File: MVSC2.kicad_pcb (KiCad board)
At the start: 4 copper layers, 68.3 x 95.1 mm, 291 parts, among them J1 USB_C-SIGNAL, J10 PWM3_OUT, J11 PWM_IN, J12 HSES, J16 ADC0, J17 ESTP0, J18 ESTP1, J19 ESTP2, J2 EXP0, J20 ESTP3, J21 ESTP4, J22 ESTP5, J23 POWER, J25 SERV0, J26 SERV1, J29 ADC1, J3 EXP1, J30 HSES, J31 HSES, J32 HSES, J4 EXPB, J5 HSES, J6 PWM0_OUT, J7 PWM1_OUT, J8 HSES, J9 PWM2_OUT, P1 STP0, P2 STP2, P3 STP4, P4 STP1, P5 STP3, P6 STP5, P9 UART, Q1 AO3400A, Q10 AO3400A, Q2 AO3400A, Q3 AO3400A, Q4 AO3400A, Q5 AO3400A, Q6 AO3400A, SW1 SKRKAEE020, SW2 SKRKAEE020, U1 XC6206P332MR, U10 TMC2208-LA-T, U11 TMC2208-LA-T, U12 TMC2208-LA-T, U13 CH912LSR, U14 CH912LSR, U2 CH912LSR, U3 STM32F411RET6, U4 CH912LSR, U5 TMC2208-LA-T, U6 TMC2208-LA-T, U7 TMC2208-LA-T, U8 CH912LSR, U9 CH912LSR, Y1 25MHZ 12pF, Y2 32.768KHz 12.5pF

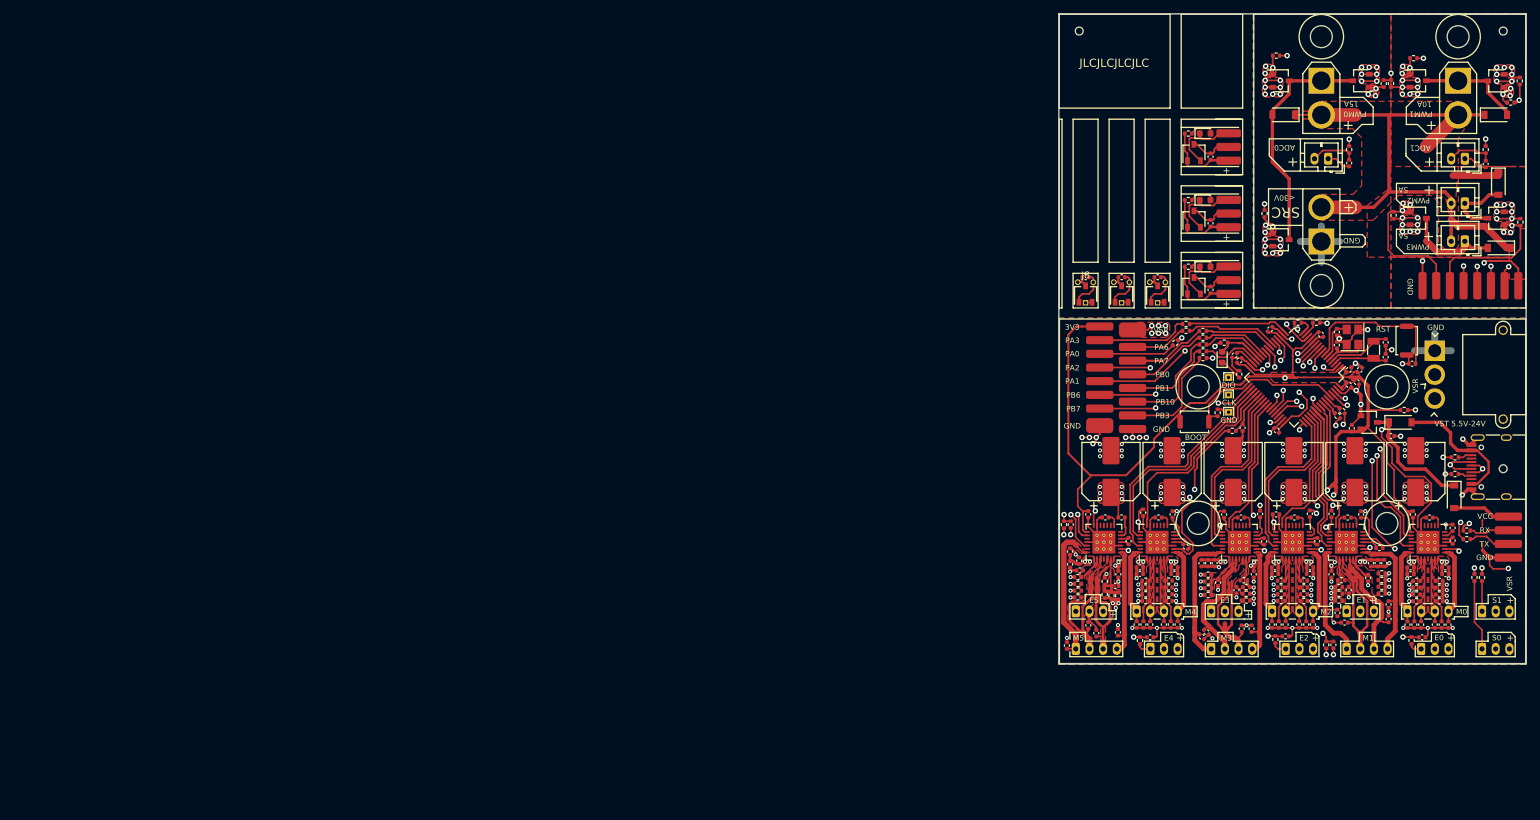
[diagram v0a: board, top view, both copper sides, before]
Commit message: going to rearrange everything
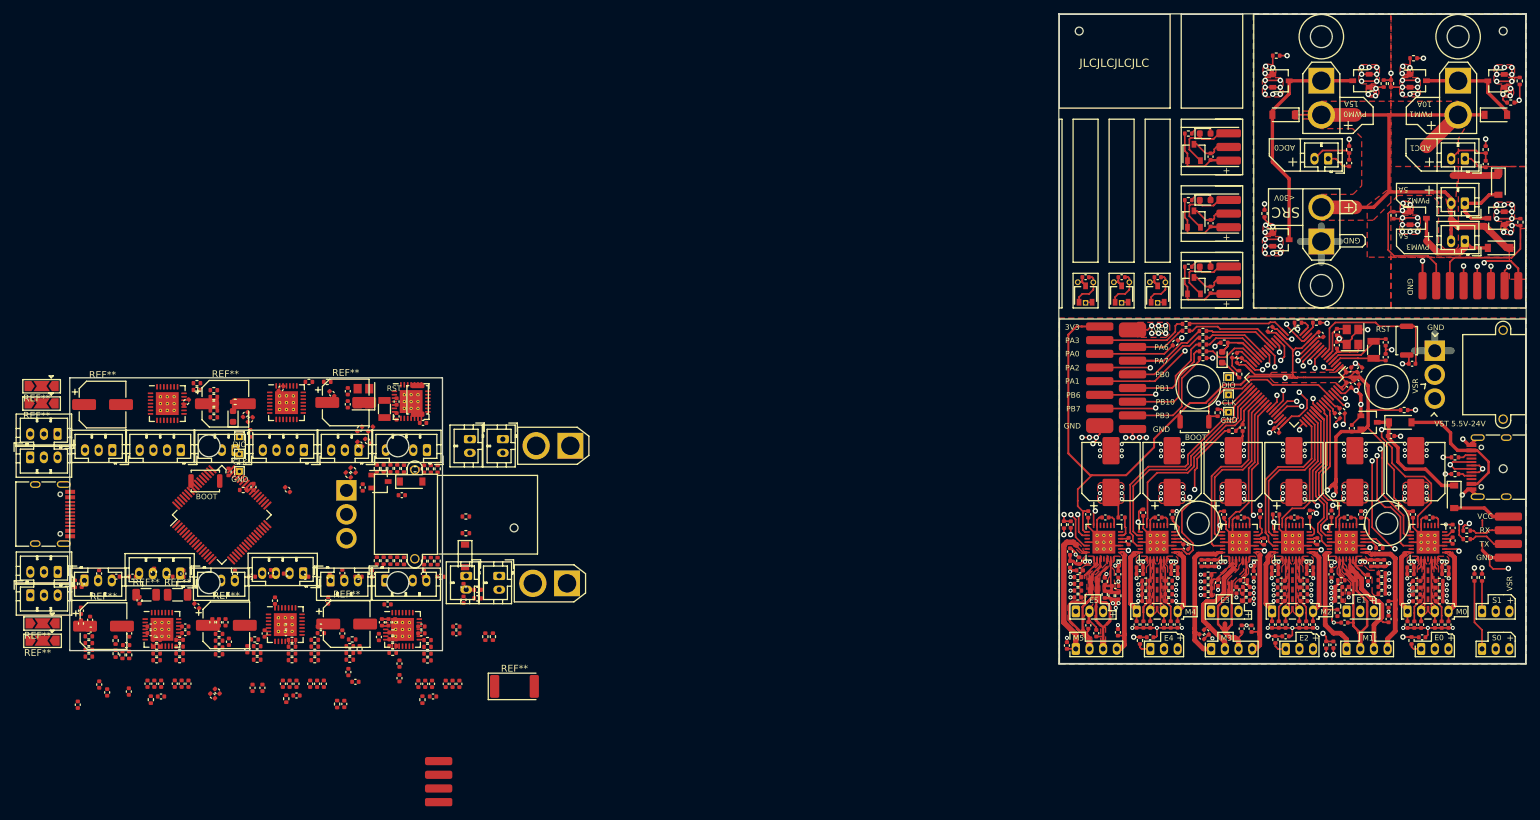
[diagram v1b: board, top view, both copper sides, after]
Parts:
- added C1: 1.0uF 25V, Capacitor_SMD:C_0402_1005Metric, F.Cu at (20.9, 145.9)
- added C10: 4.7uF 10V, Capacitor_SMD:C_0402_1005Metric, F.Cu at (-1.93, 134.1)
- added C100: 470pF 50V, Capacitor_SMD:C_0402_1005Metric, F.Cu at (-26.4, 176.5)
- added C101: 470pF 50V, Capacitor_SMD:C_0402_1005Metric, F.Cu at (-19.0, 174.6)
- added C102: 470pF 50V, Capacitor_SMD:C_0402_1005Metric, F.Cu at (14.2, 173.2)
- added C103: 470pF 50V, Capacitor_SMD:C_0402_1005Metric, F.Cu at (20.6, 172.6)
- added C104: 470pF 50V, Capacitor_SMD:C_0402_1005Metric, F.Cu at (-6.04, 174.5)
- added C105: 470pF 50V, Capacitor_SMD:C_0402_1005Metric, F.Cu at (-0.88, 174.0)
- added C106: 470pF 50V, Capacitor_SMD:C_0402_1005Metric, F.Cu at (-23.3, 173.6)
- added C107: 470pF 50V, Capacitor_SMD:C_0402_1005Metric, F.Cu at (-22.1, 174.7)
- added C108: 33nF 50V, Capacitor_SMD:C_0402_1005Metric, F.Cu at (-10.7, 166.0)
- added C109: 33nF 50V, Capacitor_SMD:C_0402_1005Metric, F.Cu at (12.2, 166.1)
- added C11: 4.7uF 10V, Capacitor_SMD:C_0402_1005Metric, F.Cu at (16.4, 136.2)
- added C110: 33nF 50V, Capacitor_SMD:C_0402_1005Metric, F.Cu at (28.9, 165.1)
- added C111: 33nF 50V, Capacitor_SMD:C_0402_1005Metric, F.Cu at (4.00, 165.1)
- added C112: 33nF 50V, Capacitor_SMD:C_0402_1005Metric, F.Cu at (0.89, 166.1)
- added C113: 33nF 50V, Capacitor_SMD:C_0402_1005Metric, F.Cu at (20.0, 164.5)
- added C114: 33nF 50V, Capacitor_SMD:C_0402_1005Metric, F.Cu at (28.9, 166.1)
- added C115: 33nF 50V, Capacitor_SMD:C_0402_1005Metric, F.Cu at (23.8, 165.1)
- added C116: 33nF 50V, Capacitor_SMD:C_0402_1005Metric, F.Cu at (-4.83, 164.5)
- added C117: 33nF 50V, Capacitor_SMD:C_0402_1005Metric, F.Cu at (-6.76, 164.5)
- added C118: 33nF 50V, Capacitor_SMD:C_0402_1005Metric, F.Cu at (19.0, 164.5)
- added C119: 33nF 50V, Capacitor_SMD:C_0402_1005Metric, F.Cu at (23.8, 166.1)
- added C12: 1.0uF 25V, Capacitor_SMD:C_0402_1005Metric, F.Cu at (15.9, 138.0)
- added C13: 100nF 16V, Capacitor_SMD:C_0402_1005Metric, F.Cu at (4.16, 157.3)
- added C14: 100nF 16V, Capacitor_SMD:C_0402_1005Metric, F.Cu at (3.28, 130.3)
- added C15: 100nF 16V, Capacitor_SMD:C_0402_1005Metric, F.Cu at (12.2, 157.3)
- added C16: 100nF 16V, Capacitor_SMD:C_0402_1005Metric, F.Cu at (14.8, 138.4)
- added C17: 100nF 16V, Capacitor_SMD:C_0402_1005Metric, F.Cu at (10.7, 131.0)
- added C18: 100nF 16V, Capacitor_SMD:C_0402_1005Metric, F.Cu at (-15.3, 157.1)
- added C19: 470pF 50V, Capacitor_SMD:C_0402_1005Metric, F.Cu at (25.5, 175.3)
- added C20: 470pF 50V, Capacitor_SMD:C_0402_1005Metric, F.Cu at (12.5, 176.4)
- added C21: 470pF 50V, Capacitor_SMD:C_0402_1005Metric, F.Cu at (5.54, 175.2)
- added C22: 470pF 50V, Capacitor_SMD:C_0402_1005Metric, F.Cu at (-0.74, 144.7)
- added C23: 470pF 50V, Capacitor_SMD:C_0402_1005Metric, F.Cu at (-14.3, 175.3)
- added C24: 470pF 50V, Capacitor_SMD:C_0402_1005Metric, F.Cu at (-25.9, 158.8)
- added C3: 1.0uF 25V, Capacitor_SMD:C_0402_1005Metric, F.Cu at (15.2, 144.7)
- added C31: 100nF 16V, Capacitor_SMD:C_0402_1005Metric, F.Cu at (28.4, 173.5)
- added C32: 100nF 16V, Capacitor_SMD:C_0402_1005Metric, F.Cu at (30.0, 159.3)
- added C33: 100nF 16V, Capacitor_SMD:C_0402_1005Metric, F.Cu at (8.55, 173.4)
- added C34: 100nF 16V, Capacitor_SMD:C_0402_1005Metric, F.Cu at (10.4, 158.0)
- added C35: 100nF 16V, Capacitor_SMD:C_0402_1005Metric, F.Cu at (-11.2, 173.4)
- added C36: 100nF 16V, Capacitor_SMD:C_0402_1005Metric, F.Cu at (-11.0, 157.3)
- added C37: 100nF 16V, Capacitor_SMD:C_0402_1005Metric, F.Cu at (24.4, 173.5)
- added C38: 100nF 16V, Capacitor_SMD:C_0402_1005Metric, F.Cu at (4.54, 173.4)
- added C39: 100nF 16V, Capacitor_SMD:C_0402_1005Metric, F.Cu at (-15.2, 173.4)
- added C40: 100nF 16V, Capacitor_SMD:C_0402_1005Metric, F.Cu at (24.2, 157.3)
- added C41: 100nF 16V, Capacitor_SMD:C_0402_1005Metric, F.Cu at (-1.21, 134.8)
- added C42: 100nF 16V, Capacitor_SMD:C_0402_1005Metric, F.Cu at (-3.45, 157.3)
- added C43: 33nF 50V, Capacitor_SMD:C_0402_1005Metric, F.Cu at (-24.6, 164.1)
- added C44: 33nF 50V, Capacitor_SMD:C_0402_1005Metric, F.Cu at (-18.9, 166.1)
- added C45: 33nF 50V, Capacitor_SMD:C_0402_1005Metric, F.Cu at (-26.0, 164.6)
- added C46: 33nF 50V, Capacitor_SMD:C_0402_1005Metric, F.Cu at (-5.79, 164.5)
- added C47: 33nF 50V, Capacitor_SMD:C_0402_1005Metric, F.Cu at (-26.0, 162.8)
- added C48: 33nF 50V, Capacitor_SMD:C_0402_1005Metric, F.Cu at (-15.8, 165.1)
- added C49: 22nF 50V, Capacitor_SMD:C_0402_1005Metric, F.Cu at (30.0, 161.2)
- added C5: 15pF, Capacitor_SMD:C_0402_1005Metric, F.Cu at (13.0, 132.6)
- added C50: 22nF 50V, Capacitor_SMD:C_0402_1005Metric, F.Cu at (10.2, 161.3)
- added C51: 22nF 50V, Capacitor_SMD:C_0402_1005Metric, F.Cu at (-9.05, 162.1)
- added C53: 4.7uF 10V, Capacitor_SMD:C_0402_1005Metric, F.Cu at (26.6, 157.8)
- added C54: 4.7uF 10V, Capacitor_SMD:C_0402_1005Metric, F.Cu at (6.83, 157.8)
- added C55: 4.7uF 10V, Capacitor_SMD:C_0402_1005Metric, F.Cu at (-13.0, 157.8)
- added C56: 470pF 50V, Capacitor_SMD:C_0402_1005Metric, F.Cu at (23.4, 173.5)
- added C57: 470pF 50V, Capacitor_SMD:C_0402_1005Metric, F.Cu at (29.4, 173.5)
- added C58: 470pF 50V, Capacitor_SMD:C_0402_1005Metric, F.Cu at (3.56, 173.4)
- added C59: 470pF 50V, Capacitor_SMD:C_0402_1005Metric, F.Cu at (9.54, 173.4)
- added C6: 15pF, Capacitor_SMD:C_0402_1005Metric, F.Cu at (13.1, 130.7)
- added C60: 470pF 50V, Capacitor_SMD:C_0402_1005Metric, F.Cu at (-16.2, 173.4)
- added C61: 470pF 50V, Capacitor_SMD:C_0402_1005Metric, F.Cu at (-10.2, 173.4)
- added C62: 470pF 50V, Capacitor_SMD:C_0402_1005Metric, F.Cu at (25.4, 173.5)
- added C63: 470pF 50V, Capacitor_SMD:C_0402_1005Metric, F.Cu at (27.4, 173.5)
- added C64: 470pF 50V, Capacitor_SMD:C_0402_1005Metric, F.Cu at (5.54, 173.4)
- added C65: 470pF 50V, Capacitor_SMD:C_0402_1005Metric, F.Cu at (7.54, 173.4)
- added C66: 470pF 50V, Capacitor_SMD:C_0402_1005Metric, F.Cu at (-14.2, 173.4)
- added C67: 470pF 50V, Capacitor_SMD:C_0402_1005Metric, F.Cu at (-12.3, 173.4)
- added C7: 15pF, Capacitor_SMD:C_0402_1005Metric, F.Cu at (20.2, 134.3)
- added C72: 100nF 16V, Capacitor_SMD:C_0402_1005Metric, F.Cu at (17.6, 166.6)
- added C73: 100nF 16V, Capacitor_SMD:C_0402_1005Metric, F.Cu at (16.6, 157.3)
- added C74: 100nF 16V, Capacitor_SMD:C_0402_1005Metric, F.Cu at (-1.65, 168.4)
- added C75: 100nF 16V, Capacitor_SMD:C_0402_1005Metric, F.Cu at (1.81, 157.3)
- added C76: 100nF 16V, Capacitor_SMD:C_0402_1005Metric, F.Cu at (-19.4, 167.8)
- added C77: 100nF 16V, Capacitor_SMD:C_0402_1005Metric, F.Cu at (-18.4, 157.8)
- added C78: 100nF 16V, Capacitor_SMD:C_0402_1005Metric, F.Cu at (14.8, 168.4)
- added C79: 100nF 16V, Capacitor_SMD:C_0402_1005Metric, F.Cu at (-4.33, 167.3)
- added C8: 15pF, Capacitor_SMD:C_0402_1005Metric, F.Cu at (20.2, 132.2)
- added C80: 100nF 16V, Capacitor_SMD:C_0402_1005Metric, F.Cu at (-24.6, 165.5)
- added C81: 100nF 16V, Capacitor_SMD:C_0402_1005Metric, F.Cu at (14.8, 136.2)
- added C82: 100nF 16V, Capacitor_SMD:C_0402_1005Metric, F.Cu at (-23.3, 157.3)
- added C83: 100nF 16V, Capacitor_SMD:C_0402_1005Metric, F.Cu at (4.24, 145.1)
- added C84: 33nF 50V, Capacitor_SMD:C_0402_1005Metric, F.Cu at (9.11, 166.0)
- added C85: 33nF 50V, Capacitor_SMD:C_0402_1005Metric, F.Cu at (-10.7, 165.1)
- added C86: 33nF 50V, Capacitor_SMD:C_0402_1005Metric, F.Cu at (-15.8, 166.0)
- added C87: 33nF 50V, Capacitor_SMD:C_0402_1005Metric, F.Cu at (18.0, 164.5)
- added C88: 33nF 50V, Capacitor_SMD:C_0402_1005Metric, F.Cu at (9.11, 165.1)
- added C89: 33nF 50V, Capacitor_SMD:C_0402_1005Metric, F.Cu at (4.00, 166.0)
- added C9: 100nF 16V, Capacitor_SMD:C_0402_1005Metric, F.Cu at (24.1, 135.3)
- added C90: 22nF 50V, Capacitor_SMD:C_0402_1005Metric, F.Cu at (18.9, 161.8)
- added C91: 22nF 50V, Capacitor_SMD:C_0402_1005Metric, F.Cu at (2.40, 161.3)
- added C92: 22nF 50V, Capacitor_SMD:C_0402_1005Metric, F.Cu at (-17.4, 161.2)
- added C93: 4.7uF 10V, Capacitor_SMD:C_0402_1005Metric, F.Cu at (14.6, 157.8)
- added C94: 4.7uF 10V, Capacitor_SMD:C_0402_1005Metric, F.Cu at (-0.97, 157.8)
- added C95: 4.7uF 10V, Capacitor_SMD:C_0402_1005Metric, F.Cu at (-20.8, 157.8)
- added C96: 470pF 50V, Capacitor_SMD:C_0402_1005Metric, F.Cu at (13.1, 171.7)
- added C97: 470pF 50V, Capacitor_SMD:C_0402_1005Metric, F.Cu at (20.6, 170.5)
- added C98: 470pF 50V, Capacitor_SMD:C_0402_1005Metric, F.Cu at (-6.72, 175.2)
- added C99: 470pF 50V, Capacitor_SMD:C_0402_1005Metric, F.Cu at (0.56, 174.0)
- added D1: B5819W, Diode_SMD:D_SOD-123, F.Cu at (22.3, 143.9)
- added D2: Blue, LED_SMD:LED_0603_1608Metric, F.Cu at (-3.73, 134.4)
- added D3: B5819W, Diode_SMD:D_SOD-123, F.Cu at (30.2, 154.8)
- added J1: USB_C-SIGNAL, Connector_USB:USB_C_Receptacle_HRO_TYPE-C-31-M-12, F.Cu at (-31.6, 148.6)
- added J16: ADC0, Connector_JST:JST_PH_B2B-PH-K_1x02_P2.00mm_Vertical, F.Cu at (30.4, 157.7)
- added J16: ADC0, Connector_JST:JST_PH_B2B-PH-K_1x02_P2.00mm_Vertical, F.Cu at (35.2, 157.7)
- added J16: ADC0, Connector_JST:JST_PH_B2B-PH-K_1x02_P2.00mm_Vertical, F.Cu at (35.7, 137.7)
- added J16: ADC0, Connector_JST:JST_PH_B2B-PH-K_1x02_P2.00mm_Vertical, F.Cu at (30.9, 137.7)
- added J17: ESTP0, Connector_JST:JST_PH_B3B-PH-K_1x03_P2.00mm_Vertical, F.Cu at (-21.4, 139.3)
- added J18: ESTP1, Connector_JST:JST_PH_B3B-PH-K_1x03_P2.00mm_Vertical, F.Cu at (10.5, 158.3)
- added J19: ESTP2, Connector_JST:JST_PH_B3B-PH-K_1x03_P2.00mm_Vertical, F.Cu at (-3.38, 139.3)
- added J20: ESTP3, Connector_JST:JST_PH_B3B-PH-K_1x03_P2.00mm_Vertical, F.Cu at (-7.46, 158.3)
- added J21: ESTP4, Connector_JST:JST_PH_B3B-PH-K_1x03_P2.00mm_Vertical, F.Cu at (14.6, 139.3)
- added J22: ESTP5, Connector_JST:JST_PH_B3B-PH-K_1x03_P2.00mm_Vertical, F.Cu at (-25.5, 158.3)
- added J23: POWER, Connector_AMASS:AMASS_MR30PW-M_1x03_P3.50mm_Horizontal, F.Cu at (12.8, 145.2)
- added J25: SERV0, Connector_JST:JST_PH_B3B-PH-K_1x03_P2.00mm_Vertical, F.Cu at (-29.4, 157.1)
- added J25: SERV0, Connector_JST:JST_PH_B3B-PH-K_1x03_P2.00mm_Vertical, F.Cu at (-29.4, 136.9)
- added J26: SERV1, Connector_JST:JST_PH_B3B-PH-K_1x03_P2.00mm_Vertical, F.Cu at (-33.4, 160.5)
- added J26: SERV1, Connector_JST:JST_PH_B3B-PH-K_1x03_P2.00mm_Vertical, F.Cu at (-33.4, 140.3)
- added J6: PWM0_OUT, Connector_AMASS:AMASS_XT30U-F_1x02_P5.0mm_Vertical, F.Cu at (45.6, 138.6)
- added J7: PWM1_OUT, Connector_AMASS:AMASS_XT30U-F_1x02_P5.0mm_Vertical, F.Cu at (45.1, 158.8)
- added P1: STP0, Connector_JST:JST_PH_B4B-PH-K_1x04_P2.00mm_Vertical, F.Cu at (18.5, 158.3)
- added P2: STP2, Connector_JST:JST_PH_B4B-PH-K_1x04_P2.00mm_Vertical, F.Cu at (6.53, 157.3)
- added P3: STP4, Connector_JST:JST_PH_B4B-PH-K_1x04_P2.00mm_Vertical, F.Cu at (-11.5, 157.3)
- added P4: STP1, Connector_JST:JST_PH_B4B-PH-K_1x04_P2.00mm_Vertical, F.Cu at (-11.4, 139.3)
- added P5: STP3, Connector_JST:JST_PH_B4B-PH-K_1x04_P2.00mm_Vertical, F.Cu at (6.62, 139.3)
- added P6: STP5, Connector_JST:JST_PH_B4B-PH-K_1x04_P2.00mm_Vertical, F.Cu at (24.6, 139.3)
- added P9: UART, Connector_JST:JST_PH_B4B-PH-K_1x04_P2.00mm_Vertical, F.Cu at (26.3, 190.8)
- added R100: 330R, Resistor_SMD:R_0402_1005Metric, F.Cu at (-2.25, 145.1)
- added R101: 330R, Resistor_SMD:R_0402_1005Metric, F.Cu at (-15.8, 175.8)
- added R102: 330R, Resistor_SMD:R_0402_1005Metric, F.Cu at (-26.9, 158.8)
- added R103: 330R, Resistor_SMD:R_0402_1005Metric, F.Cu at (33.2, 166.6)
- added R104: 330R, Resistor_SMD:R_0402_1005Metric, F.Cu at (34.3, 166.6)
- added R17: 33k, Resistor_SMD:R_0402_1005Metric, F.Cu at (-4.39, 142.5)
- added R29: 5.1k, Resistor_SMD:R_0402_1005Metric, F.Cu at (-1.24, 136.8)
- added R3: 5.1k, Resistor_SMD:R_0402_1005Metric, F.Cu at (30.3, 151.4)
- added R30: 33k, Resistor_SMD:R_0402_1005Metric, F.Cu at (-3.42, 132.2)
- added R32: 330R, Resistor_SMD:R_0402_1005Metric, F.Cu at (-9.02, 130.5)
- added R33: 330R, Resistor_SMD:R_0402_1005Metric, F.Cu at (-6.54, 130.5)
- added R34: 330R, Resistor_SMD:R_0402_1005Metric, F.Cu at (-6.54, 131.5)
- added R35: 330R, Resistor_SMD:R_0402_1005Metric, F.Cu at (-6.54, 132.5)
- added R36: 330R, Resistor_SMD:R_0402_1005Metric, F.Cu at (-6.54, 133.5)
- added R37: 330R, Resistor_SMD:R_0402_1005Metric, F.Cu at (-6.54, 134.5)
- added R38: 330R, Resistor_SMD:R_0402_1005Metric, F.Cu at (-9.02, 129.5)
- added R4: 5.1k, Resistor_SMD:R_0402_1005Metric, F.Cu at (30.3, 149.0)
- added R40: 330R, Resistor_SMD:R_0402_1005Metric, F.Cu at (7.36, 129.3)
- added R41: 330R, Resistor_SMD:R_0402_1005Metric, F.Cu at (10.0, 129.3)
- added R42: 330R, Resistor_SMD:R_0402_1005Metric, F.Cu at (-10.6, 132.2)
- added R43: 330R, Resistor_SMD:R_0402_1005Metric, F.Cu at (13.1, 142.9)
- added R44: 330R, Resistor_SMD:R_0402_1005Metric, F.Cu at (13.8, 142.2)
- added R45: 10k, Resistor_SMD:R_0402_1005Metric, F.Cu at (22.9, 142.1)
- added R47: 1R, Resistor_SMD:R_0402_1005Metric, F.Cu at (24.7, 168.1)
- added R48: 1R, Resistor_SMD:R_0402_1005Metric, F.Cu at (24.7, 167.1)
- added R49: 1R, Resistor_SMD:R_0402_1005Metric, F.Cu at (24.7, 170.0)
- added R50: 1R, Resistor_SMD:R_0402_1005Metric, F.Cu at (24.7, 169.0)
- added R51: 1R, Resistor_SMD:R_0402_1005Metric, F.Cu at (17.3, 142.0)
- added R51: 1R, Resistor_SMD:R_0402_1005Metric, F.Cu at (21.3, 142.0)
- added R51: 1R, Resistor_SMD:R_0402_1005Metric, F.Cu at (17.3, 155.4)
- added R51: 1R, Resistor_SMD:R_0402_1005Metric, F.Cu at (21.3, 155.5)
- added R52: 1R, Resistor_SMD:R_0402_1005Metric, F.Cu at (20.3, 142.0)
- added R52: 1R, Resistor_SMD:R_0402_1005Metric, F.Cu at (26.2, 142.0)
- added R52: 1R, Resistor_SMD:R_0402_1005Metric, F.Cu at (20.3, 155.4)
- added R52: 1R, Resistor_SMD:R_0402_1005Metric, F.Cu at (26.2, 155.5)
- added R53: 1R, Resistor_SMD:R_0402_1005Metric, F.Cu at (19.3, 142.0)
- added R53: 1R, Resistor_SMD:R_0402_1005Metric, F.Cu at (25.2, 142.0)
- added R53: 1R, Resistor_SMD:R_0402_1005Metric, F.Cu at (19.3, 155.4)
- added R53: 1R, Resistor_SMD:R_0402_1005Metric, F.Cu at (25.2, 155.5)
- added R54: 1R, Resistor_SMD:R_0402_1005Metric, F.Cu at (24.2, 142.0)
- added R54: 1R, Resistor_SMD:R_0402_1005Metric, F.Cu at (18.3, 142.0)
- added R54: 1R, Resistor_SMD:R_0402_1005Metric, F.Cu at (18.3, 155.4)
- added R54: 1R, Resistor_SMD:R_0402_1005Metric, F.Cu at (24.2, 155.5)
- added R55: 1R, Resistor_SMD:R_0402_1005Metric, F.Cu at (4.89, 168.0)
- added R56: 1R, Resistor_SMD:R_0402_1005Metric, F.Cu at (4.89, 167.0)
- added R57: 1R, Resistor_SMD:R_0402_1005Metric, F.Cu at (4.89, 169.0)
- added R58: 1R, Resistor_SMD:R_0402_1005Metric, F.Cu at (4.89, 170.0)
- added R59: 1R, Resistor_SMD:R_0402_1005Metric, F.Cu at (8.21, 168.0)
- added R60: 1R, Resistor_SMD:R_0402_1005Metric, F.Cu at (8.21, 169.0)
- added R61: 1R, Resistor_SMD:R_0402_1005Metric, F.Cu at (8.21, 170.0)
- added R62: 1R, Resistor_SMD:R_0402_1005Metric, F.Cu at (8.21, 167.0)
- added R63: 1R, Resistor_SMD:R_0402_1005Metric, F.Cu at (-14.9, 168.0)
- added R64: 1R, Resistor_SMD:R_0402_1005Metric, F.Cu at (-14.9, 167.0)
- added R65: 1R, Resistor_SMD:R_0402_1005Metric, F.Cu at (-14.9, 169.0)
- added R66: 1R, Resistor_SMD:R_0402_1005Metric, F.Cu at (-14.9, 170.0)
- added R67: 1R, Resistor_SMD:R_0402_1005Metric, F.Cu at (-11.6, 168.0)
- added R68: 1R, Resistor_SMD:R_0402_1005Metric, F.Cu at (-11.6, 169.0)
- added R69: 1R, Resistor_SMD:R_0402_1005Metric, F.Cu at (-11.6, 170.0)
- added R7: 330R, Resistor_SMD:R_0402_1005Metric, F.Cu at (32.0, 160.9)
- added R70: 1R, Resistor_SMD:R_0402_1005Metric, F.Cu at (-11.6, 167.0)
- added R73: 1R, Resistor_SMD:R_0402_1005Metric, F.Cu at (13.7, 167.0)
- added R74: 1R, Resistor_SMD:R_0402_1005Metric, F.Cu at (13.3, 168.9)
- added R75: 1R, Resistor_SMD:R_0402_1005Metric, F.Cu at (13.3, 169.9)
- added R76: 1R, Resistor_SMD:R_0402_1005Metric, F.Cu at (13.3, 167.9)
- added R77: 1R, Resistor_SMD:R_0402_1005Metric, F.Cu at (19.6, 167.9)
- added R78: 1R, Resistor_SMD:R_0402_1005Metric, F.Cu at (19.6, 165.9)
- added R79: 1R, Resistor_SMD:R_0402_1005Metric, F.Cu at (19.6, 168.9)
- added R8: 330R, Resistor_SMD:R_0402_1005Metric, F.Cu at (32.0, 159.7)
- added R80: 1R, Resistor_SMD:R_0402_1005Metric, F.Cu at (19.6, 166.9)
- added R81: 1R, Resistor_SMD:R_0402_1005Metric, F.Cu at (-5.78, 167.1)
- added R82: 1R, Resistor_SMD:R_0402_1005Metric, F.Cu at (-5.78, 168.1)
- added R83: 1R, Resistor_SMD:R_0402_1005Metric, F.Cu at (-5.78, 169.1)
- added R84: 1R, Resistor_SMD:R_0402_1005Metric, F.Cu at (-5.78, 166.2)
- added R85: 1R, Resistor_SMD:R_0402_1005Metric, F.Cu at (-0.20, 168.9)
- added R86: 1R, Resistor_SMD:R_0402_1005Metric, F.Cu at (-0.56, 167.0)
- added R87: 1R, Resistor_SMD:R_0402_1005Metric, F.Cu at (-0.20, 168.0)
- added R88: 1R, Resistor_SMD:R_0402_1005Metric, F.Cu at (-0.20, 169.9)
- added R89: 1R, Resistor_SMD:R_0402_1005Metric, F.Cu at (-24.8, 166.5)
- added R90: 1R, Resistor_SMD:R_0402_1005Metric, F.Cu at (-24.8, 167.5)
- added R91: 1R, Resistor_SMD:R_0402_1005Metric, F.Cu at (-24.8, 169.5)
- added R92: 1R, Resistor_SMD:R_0402_1005Metric, F.Cu at (-24.8, 168.5)
- added R93: 1R, Resistor_SMD:R_0402_1005Metric, F.Cu at (-20.9, 167.1)
- added R94: 1R, Resistor_SMD:R_0402_1005Metric, F.Cu at (-18.9, 169.2)
- added R95: 1R, Resistor_SMD:R_0402_1005Metric, F.Cu at (-19.9, 169.2)
- added R96: 1R, Resistor_SMD:R_0402_1005Metric, F.Cu at (-20.9, 169.0)
- added R97: 330R, Resistor_SMD:R_0402_1005Metric, F.Cu at (24.0, 175.8)
- added R98: 330R, Resistor_SMD:R_0402_1005Metric, F.Cu at (11.5, 176.4)
- added R99: 330R, Resistor_SMD:R_0402_1005Metric, F.Cu at (4.05, 175.6)
- added REF**: R_1206_3216Metric, Resistor_SMD:R_1206_3216Metric, F.Cu at (-11.8, 160.4)
- added REF**: CP_Elec_6.3x7.7, Capacitor_SMD:CP_Elec_6.3x7.7, F.Cu at (-22.8, 132.6)
- added REF**: CP_Elec_6.3x7.7, Capacitor_SMD:CP_Elec_6.3x7.7, F.Cu at (-4.71, 164.9)
- added REF**: CP_Elec_6.3x7.7, Capacitor_SMD:CP_Elec_6.3x7.7, F.Cu at (-22.7, 165.0)
- added REF**: CP_Elec_6.3x7.7, Capacitor_SMD:CP_Elec_6.3x7.7, F.Cu at (12.9, 164.7)
- added REF**: MountingHole_3.2mm_M3, MountingHole:MountingHole_3.2mm_M3, F.Cu at (20.4, 138.7)
- added REF**: ToolingHole, MountingHole:MountingHole_3.2mm_M3, F.Cu at (35.4, 150.7)
- added REF**: MountingHole_3.2mm_M3, MountingHole:MountingHole_3.2mm_M3, F.Cu at (20.4, 158.7)
- added REF**: MountingHole_3.2mm_M3, MountingHole:MountingHole_3.2mm_M3, F.Cu at (-7.24, 158.7)
- added REF**: MountingHole_3.2mm_M3, MountingHole:MountingHole_3.2mm_M3, F.Cu at (-7.24, 138.7)
- added REF**: R_1206_3216Metric, Resistor_SMD:R_1206_3216Metric, F.Cu at (-16.4, 160.4)
- added REF**: D_2512_6332Metric, Diode_SMD:D_2512_6332Metric, F.Cu at (37.4, 173.8)
- added REF**: SolderJumper-3_P2.0mm_Open_TrianglePad1.0x1.5mm, Jumper:SolderJumper-3_P2.0mm_Open_TrianglePad1.0x1.5mm, F.Cu at (-31.6, 167.1)
- added REF**: SolderJumper-3_P2.0mm_Open_TrianglePad1.0x1.5mm, Jumper:SolderJumper-3_P2.0mm_Open_TrianglePad1.0x1.5mm, F.Cu at (-31.6, 164.6)
- added REF**: SolderJumper-3_P2.0mm_Open_TrianglePad1.0x1.5mm, Jumper:SolderJumper-3_P2.0mm_Open_TrianglePad1.0x1.5mm, F.Cu at (-31.7, 129.9)
- added REF**: SolderJumper-3_P2.0mm_Open_TrianglePad1.0x1.5mm, Jumper:SolderJumper-3_P2.0mm_Open_TrianglePad1.0x1.5mm, F.Cu at (-31.7, 132.4)
- added REF**: CP_Elec_6.3x7.7, Capacitor_SMD:CP_Elec_6.3x7.7, F.Cu at (12.7, 132.3)
- added REF**: CP_Elec_6.3x7.7, Capacitor_SMD:CP_Elec_6.3x7.7, F.Cu at (-4.86, 132.5)
- added SW1: SKRKAEE020, Button_Switch_SMD:SW_Push_SPST_NO_Alps_SKRK, F.Cu at (23.3, 131.9)
- added SW2: SKRKAEE020, Button_Switch_SMD:SW_Push_SPST_NO_Alps_SKRK, F.Cu at (-7.78, 143.8)
- added TP1: SWD_DIO, TestPoint:TestPoint_THTPad_1.0x1.0mm_Drill0.5mm, F.Cu at (-2.80, 137.3)
- added TP2: SWD_CLK, TestPoint:TestPoint_THTPad_1.0x1.0mm_Drill0.5mm, F.Cu at (-2.80, 139.9)
- added TP3: SWD_GND, TestPoint:TestPoint_THTPad_1.0x1.0mm_Drill0.5mm, F.Cu at (-2.80, 142.4)
- added U1: XC6206P332MR, Package_TO_SOT_SMD:SOT-23W, F.Cu at (17.8, 143.9)
- added U10: TMC2208-LA-T, Package_DFN_QFN:QFN-28-1EP_5x5mm_P0.5mm_EP3.35x3.35mm_ThermalVias, F.Cu at (22.3, 132.2)
- added U11: TMC2208-LA-T, Package_DFN_QFN:QFN-28-1EP_5x5mm_P0.5mm_EP3.35x3.35mm_ThermalVias, F.Cu at (4.08, 132.3)
- added U12: TMC2208-LA-T, Package_DFN_QFN:QFN-28-1EP_5x5mm_P0.5mm_EP3.35x3.35mm_ThermalVias, F.Cu at (-14.1, 165.5)
- added U3: STM32F411RET6, Package_QFP:LQFP-64_10x10mm_P0.5mm, F.Cu at (-5.38, 148.7)
- added U5: TMC2208-LA-T, Package_DFN_QFN:QFN-28-1EP_5x5mm_P0.5mm_EP3.35x3.35mm_ThermalVias, F.Cu at (3.90, 164.8)
- added U6: TMC2208-LA-T, Package_DFN_QFN:QFN-28-1EP_5x5mm_P0.5mm_EP3.35x3.35mm_ThermalVias, F.Cu at (21.1, 165.5)
- added U7: TMC2208-LA-T, Package_DFN_QFN:QFN-28-1EP_5x5mm_P0.5mm_EP3.35x3.35mm_ThermalVias, F.Cu at (-13.3, 132.5)
- added Y1: 25MHZ 12pF, Crystal:Crystal_SMD_3225-4Pin_3.2x2.5mm, F.Cu at (15.3, 131.4)
- added Y2: 32.768KHz 12.5pF, Crystal:Crystal_SMD_3215-2Pin_3.2x1.5mm, F.Cu at (18.4, 133.3)
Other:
- board size 68.3 x 95.1 mm -> 213 x 95.1 mm
